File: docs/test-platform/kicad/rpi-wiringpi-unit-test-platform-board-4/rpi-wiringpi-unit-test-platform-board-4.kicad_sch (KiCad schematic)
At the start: 5 parts, among them J1 JST_IN_PWR, J2 JST_IN_I2C, M1 DS3231_0x68+AT24C32_0x57, M2 BMP180_0x77, M3 SSD1306_0x3c

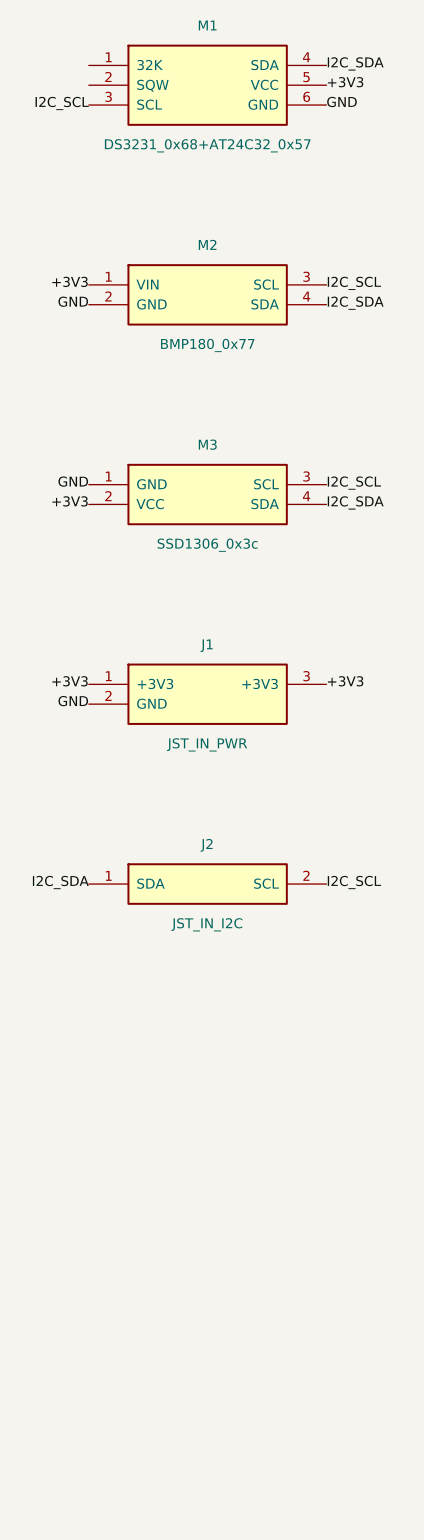
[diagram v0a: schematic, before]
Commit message: Added KiCAD board 4
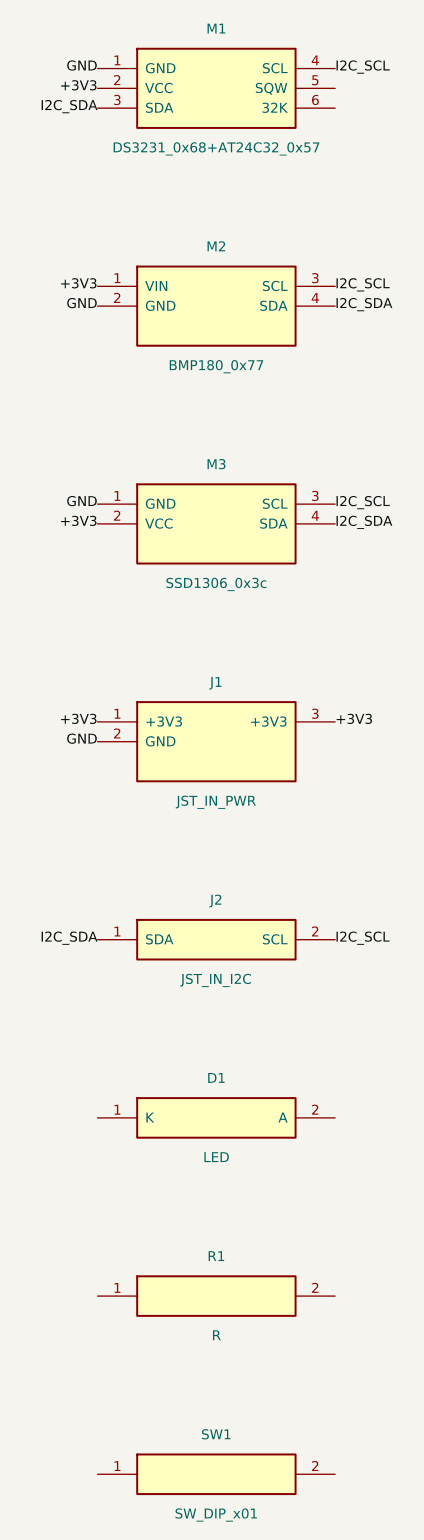
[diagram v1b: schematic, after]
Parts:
- added D1: LED, rpi-wiringpi-unit-test-platform-board-4:D1, symbol rpi-wiringpi-unit-test-platform-board-4:D1
- added R1: R, rpi-wiringpi-unit-test-platform-board-4:R1, symbol rpi-wiringpi-unit-test-platform-board-4:R1
- added SW1: SW_DIP_x01, rpi-wiringpi-unit-test-platform-board-4:SW1, symbol rpi-wiringpi-unit-test-platform-board-4:SW1
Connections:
- net +3V3: now also M1.2 (VCC); no longer M1.5 (VCC)
- net GND: now also M1.1 (GND); no longer M1.6 (GND)
- net I2C_SCL: now also M1.4 (SCL); no longer M1.3 (SCL)
- net I2C_SDA: now also M1.3 (SDA); no longer M1.4 (SDA)
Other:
- moved on the sheet: J1, J2, M1, M2, M3
